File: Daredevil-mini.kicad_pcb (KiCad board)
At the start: 2 copper layers, 45.9 x 21 mm, 55 parts, among them J1 USB_A, SW1 KMR221GLFS, Y1 ABM8-272-T3

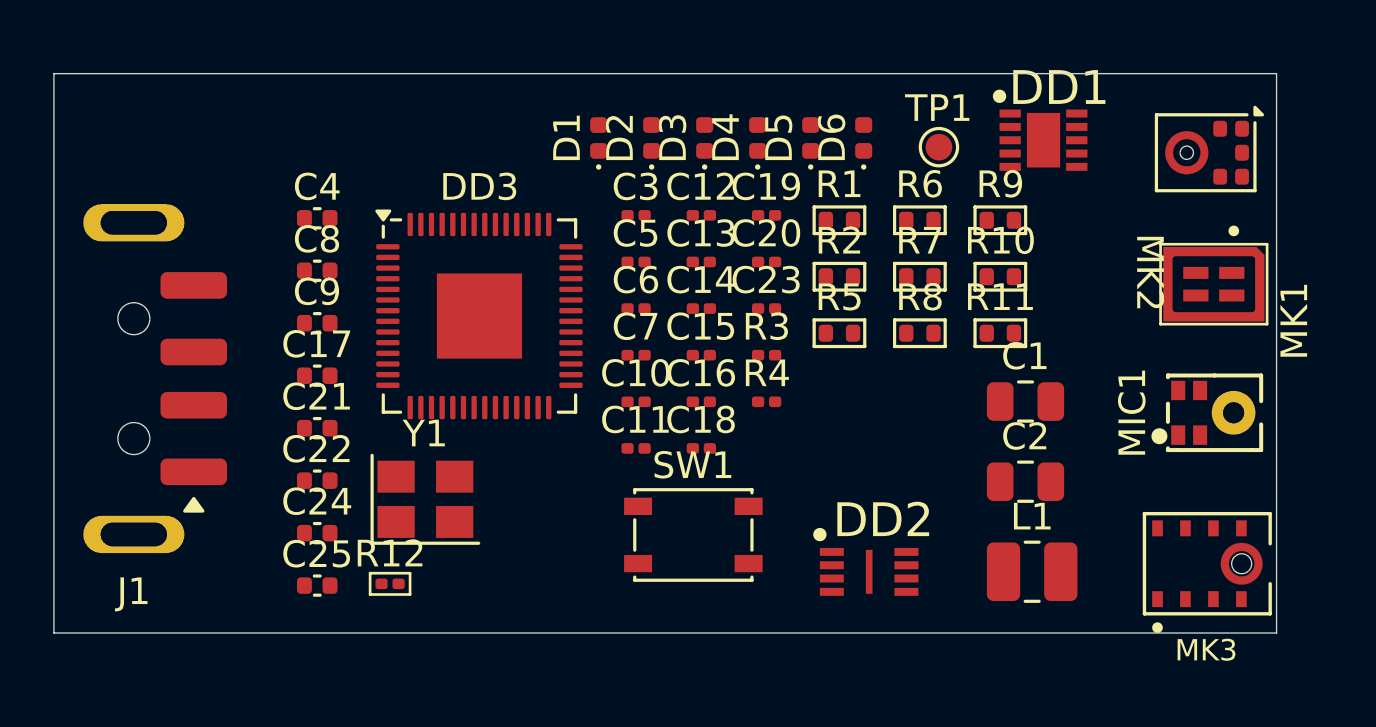
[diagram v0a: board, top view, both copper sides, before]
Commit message: udp PCB
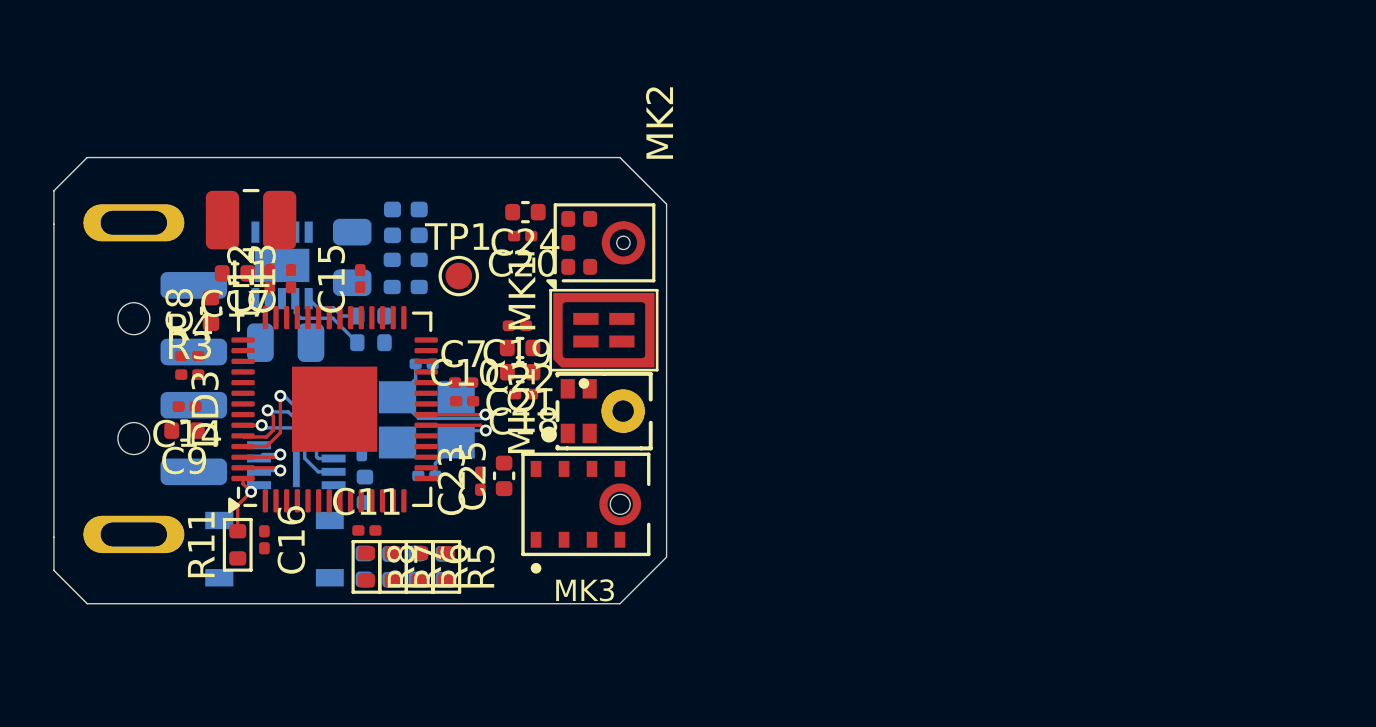
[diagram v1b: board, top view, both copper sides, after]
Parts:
- removed R12: 0R, PCM_Resistor_SMD_AKL:R_0201_0603Metric
- C1, C2, C3, C4, C5, C6, D1, D2, D3, D4, D5, D6, DD1, DD2, J1, R1, R10, R2, R9, SW1, Y1: moved to B.Cu
- moved L1 32.2 mm to (127.4, 96.6), turned to 180 degrees
- moved R11 29.7 mm to (126.9, 108.8), turned to 90 degrees
- moved DD1 29.0 mm to (128.6, 98.3), turned to -90 degrees
- moved C2 28.3 mm to (128.7, 101.2)
- moved C1 25.8 mm to (131.2, 98.0), turned to -90 degrees
- moved MK3 23.4 mm to (140.0, 107.3)
- moved MK1 23.0 mm to (140.6, 100.7), turned to 90 degrees
- moved MIC1 22.9 mm to (140.6, 103.8)
- moved R6 22.8 mm to (133.7, 109.6), turned to -90 degrees
- moved R10 22.8 mm to (132.7, 98.6), turned to 90 degrees
- moved MK2 22.8 mm to (140.7, 97.5), turned to 90 degrees
- moved R7 22.6 mm to (132.7, 109.6), turned to -90 degrees
- moved R8 22.6 mm to (131.7, 109.6), turned to -90 degrees
- moved R9 21.9 mm to (133.7, 98.6), turned to 90 degrees
- moved DD2 21.9 mm to (129.1, 105.8)
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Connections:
- MK1 pad 2: Net-(MK1-LR) -> Earth
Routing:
- net Net-(DD3-XOUT): track 0.00 -> 7.44 mm, vias 0 -> 1
- net Net-(DD2-DI(IO0)): track 0.00 -> 5.76 mm, vias 0 -> 1
- net Net-(DD2-CLK): track 0.00 -> 5.68 mm, vias 0 -> 1
- net Net-(DD3-XIN): track 0.00 -> 5.19 mm, vias 0 -> 1
- net Net-(DD2-IO3): track 0.00 -> 4.57 mm, vias 0 -> 1
- net Net-(DD1-PS): track 0.00 -> 3.32 mm
- net Net-(DD2-~{CS}): track 0.00 -> 2.71 mm, vias 0 -> 1
- net Net-(DD2-IO2): track 0.00 -> 2.30 mm, vias 0 -> 1
- net Net-(DD2-DO(IO1)): track 0.00 -> 2.26 mm, vias 0 -> 1
- net Net-(DD1-EN): track 0.00 -> 2.10 mm
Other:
- board size 45.9 x 21 mm -> 23 x 16.8 mm

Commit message: rev0 ready
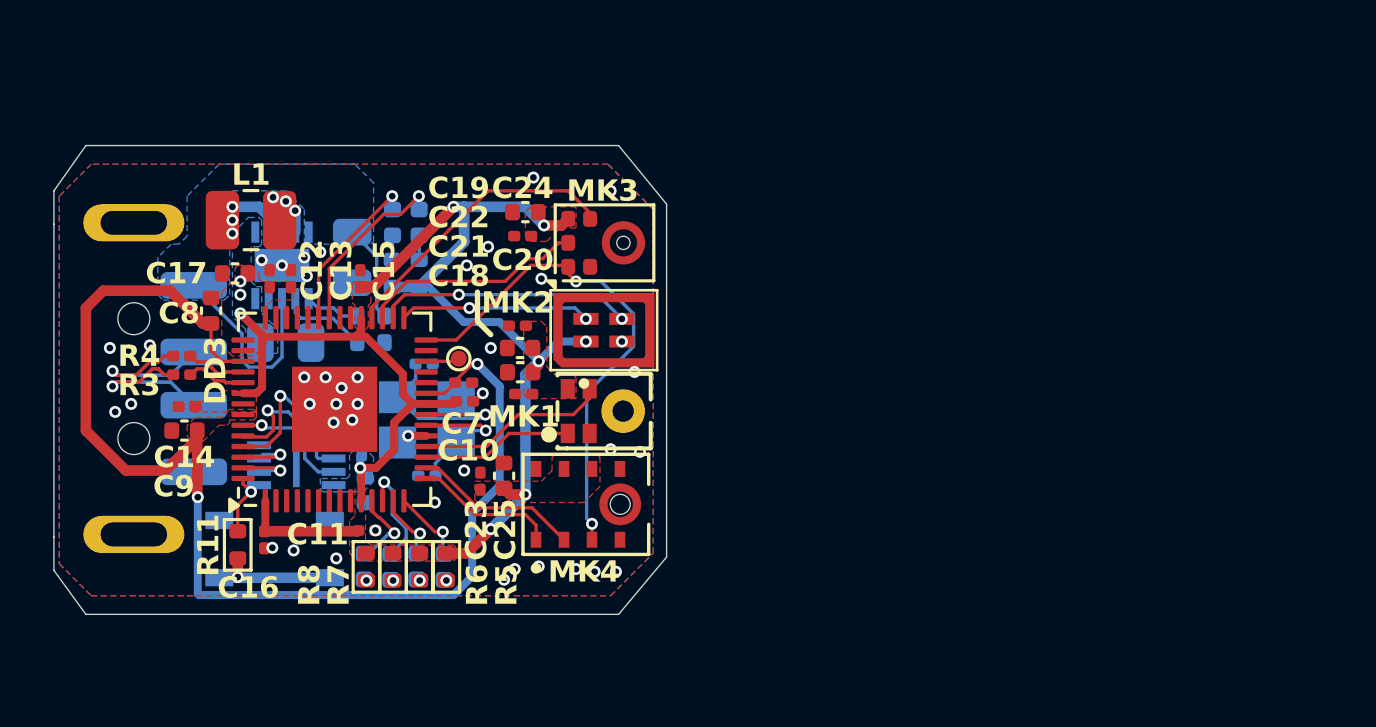
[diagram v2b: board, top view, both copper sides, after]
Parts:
- moved TP1 3.10 mm to (135.2, 101.8)
- moved R3 0.30 mm to (124.8, 102.4)
- moved R4 0.30 mm to (124.8, 101.7)
- turned D1 to -90 degrees
- renumbered MIC1 to MK1, MK1 to MK2, MK2 to MK3, MK3 to MK4
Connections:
- DD3 pad 11: unconnected-(DD3-GPIO8-Pad11) -> LVL_LED_4
- DD3 pad 12: SPH0645_WS -> LVL_LED_3
- DD3 pad 13: DAT3 -> LVL_LED_2
- DD3 pad 14: CLK3 -> LVL_LED_1
- DD3 pad 15: unconnected-(DD3-GPIO12-Pad15) -> CLK2
- DD3 pad 16: unconnected-(DD3-GPIO13-Pad16) -> DAT2
- DD3 pad 28: unconnected-(DD3-GPIO17-Pad28) -> SPH0645_WS
- DD3 pad 29: unconnected-(DD3-GPIO18-Pad29) -> DAT1
- DD3 pad 30: LVL_LED_1 -> CLK1
- DD3 pad 31: LVL_LED_2 -> DAT3
- DD3 pad 32: LVL_LED_3 -> CLK3
- DD3 pad 34: LVL_LED_4 -> unconnected-(DD3-GPIO22-Pad34)
- DD3 pad 4: DAT1 -> unconnected-(DD3-GPIO2-Pad4)
- DD3 pad 5: CLK1 -> unconnected-(DD3-GPIO3-Pad5)
- DD3 pad 7: INMP441_WS -> unconnected-(DD3-GPIO5-Pad7)
- DD3 pad 8: DAT2 -> unconnected-(DD3-GPIO6-Pad8)
- DD3 pad 9: CLK2 -> unconnected-(DD3-GPIO7-Pad9)
- MK4 pad 3: INMP441_WS -> SPH0645_WS
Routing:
- net +3.3V: track 0.00 -> 58.3 mm, vias 0 -> 10
- net +1.1V: track 0.00 -> 46.0 mm, vias 0 -> 2
- net SPH0645_WS: track 0.00 -> 19.1 mm, vias 0 -> 2
- net +5V: track 0.00 -> 11.2 mm
- net CLK3: track 0.00 -> 11.0 mm
- net CLK1: track 0.00 -> 9.57 mm, vias 0 -> 2
- net DAT3: track 0.00 -> 8.39 mm
- net CLK4: track 0.00 -> 7.24 mm
- net DAT1: track 0.00 -> 7.15 mm, vias 0 -> 2
- net STATUS_LED_1: track 0.00 -> 6.83 mm, vias 0 -> 1
- net DAT2: track 0.00 -> 6.29 mm
- net STATUS_LED_2: track 0.00 -> 6.21 mm, vias 0 -> 1
- net USB+: track 0.00 -> 6.12 mm, vias 0 -> 1
- net USB-: track 0.00 -> 6.12 mm, vias 0 -> 1
- net DAT4: track 0.00 -> 5.68 mm
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- added copper zone on F.Cu, net +1.1V
- added copper zone on B.Cu, net +3.3V
- added copper zone on F.Cu, net +3.3V
- added copper zone on B.Cu, net +5V
- added copper zone on B.Cu, net Earth
- added copper zone on F.Cu, net Earth
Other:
- board size 23 x 16.8 mm -> 23 x 17.6 mm
- board text added: "@madjogger"
- board text added: "Daredevil-mini"
